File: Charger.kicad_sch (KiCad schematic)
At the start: 86 parts, among them J23 Conn_02x07_Odd_Even, Q6 BSC0702LS, Q7 BSC0702LS, Q8 BSC0702LS, Q9 BSC0702LS, U2 LV2862XDDC, U27 BQ25756RRVR

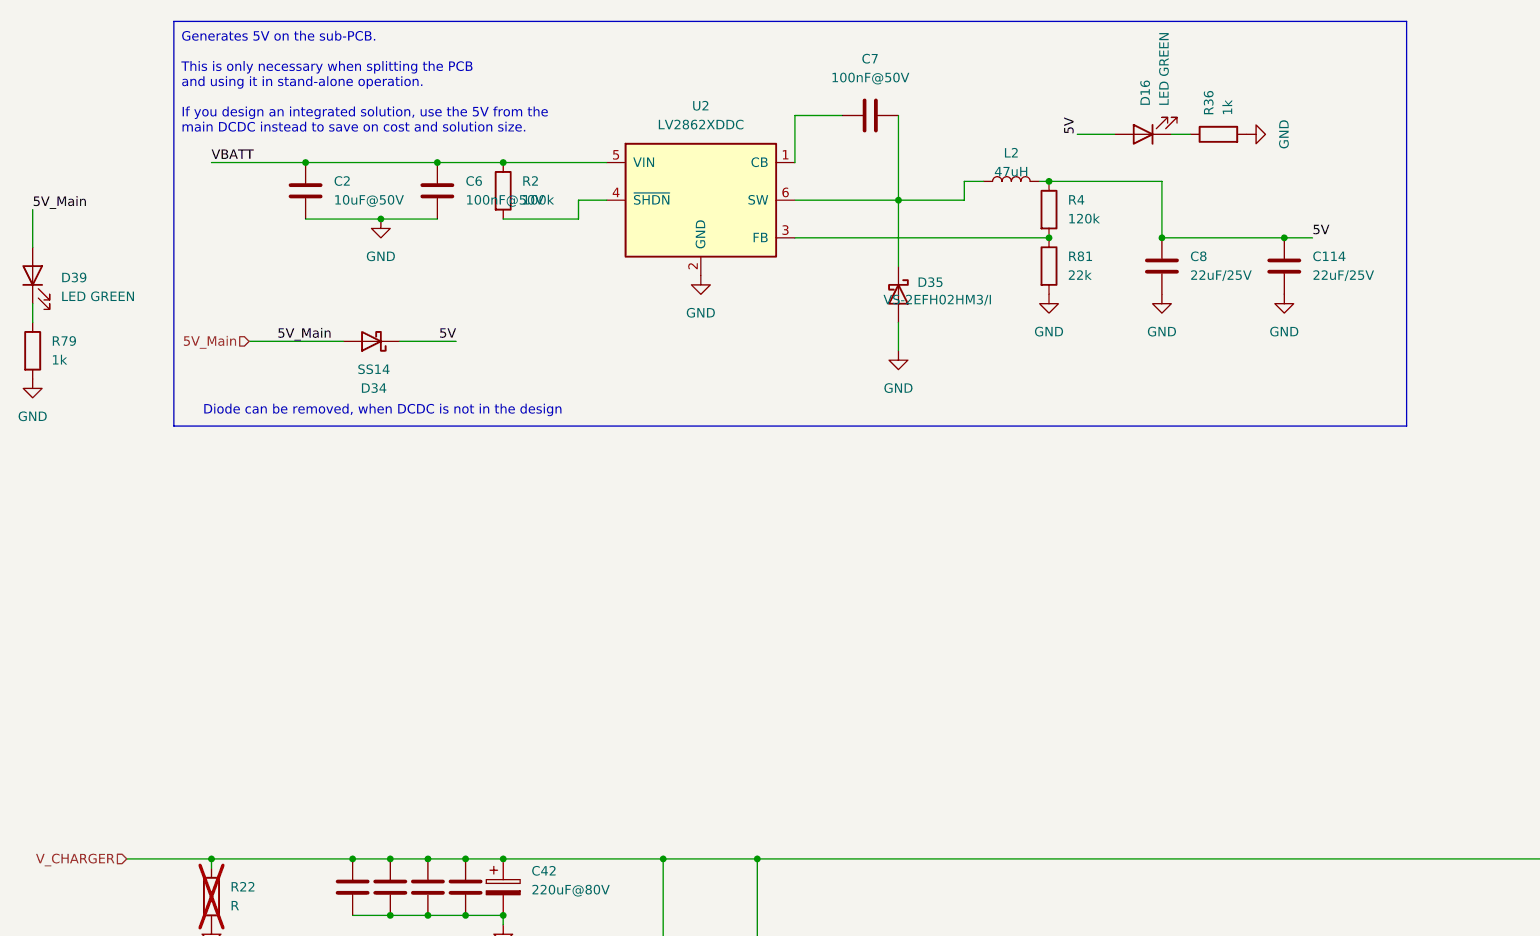
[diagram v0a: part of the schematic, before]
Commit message: wip
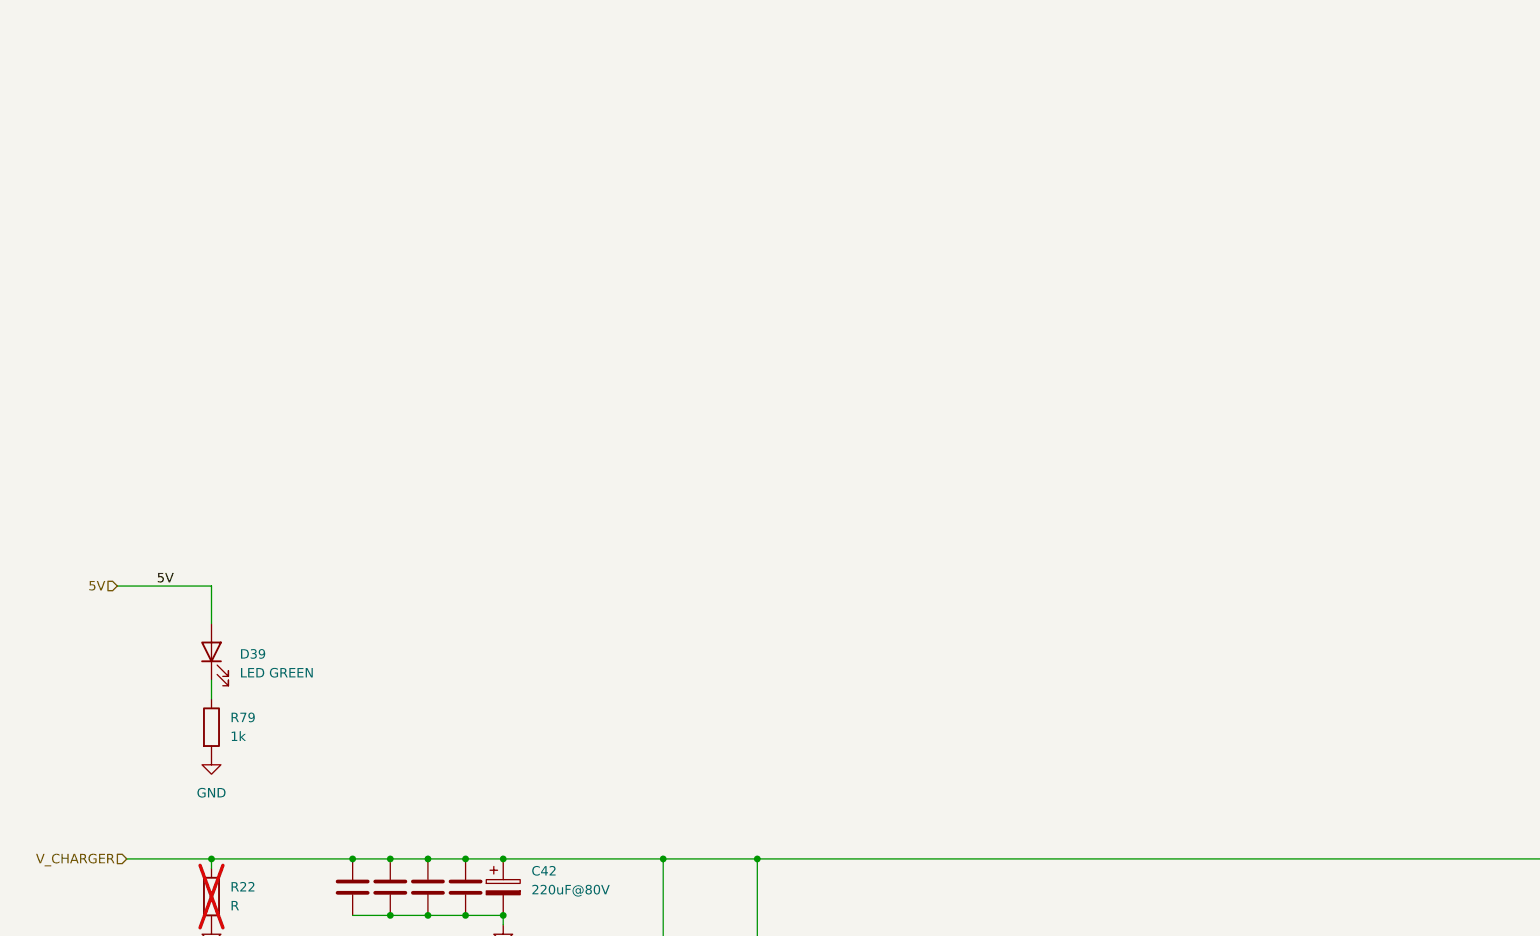
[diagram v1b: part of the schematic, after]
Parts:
- removed C114, C8: 22uF/25V, Capacitor_SMD:C_0805_2012Metric, symbol Device:C
- removed C2: 10uF@50V, Capacitor_SMD:C_1206_3216Metric, symbol Device:C
- removed C6, C7: 100nF@50V, Capacitor_SMD:C_0402_1005Metric, symbol Device:C
- removed D16: LED GREEN, LED_SMD:LED_0805_2012Metric, symbol Device:LED
- removed D34: SS14, Diode_SMD:D_SMA, symbol Diode:SS14
- removed D35: VS-2EFH02HM3/I, Diode_SMD:D_SMF, symbol Device:D_Schottky
- removed L2: 47uH, Inductor_SMD:L_Sunlord_SWPA5040S, symbol Device:L
- removed R2: 100k, Resistor_SMD:R_0402_1005Metric, symbol Device:R
- removed R36: 1k, Resistor_SMD:R_0805_2012Metric, symbol Device:R
- removed R4: 120k, Resistor_SMD:R_0603_1608Metric, symbol Device:R
- removed R81: 22k, Resistor_SMD:R_0603_1608Metric, symbol Device:R
- removed U2: LV2862XDDC, Package_TO_SOT_SMD:SOT-23-6, symbol Regulator_Switching:LV2862XDDC
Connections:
- net 5V_Main is gone; now on net 5V: D39.2 (A)
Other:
- note removed: "Diode can be removed, when DCDC is not in the design"
- note removed: "Generates 5V on the sub-PCB. This is only necessary when splitting the PCB and using it in stand-alone operation. If you design an integrated solution, use the 5V from the main DCDC instead to save on cost and solution size."
- moved on the sheet: D39, R79

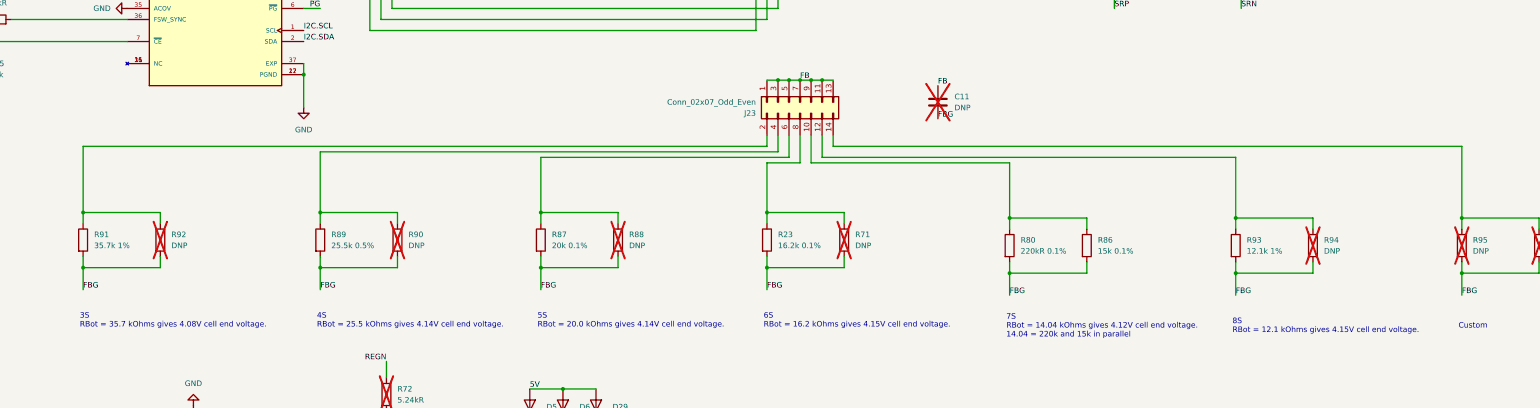
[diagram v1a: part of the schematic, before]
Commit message: wip
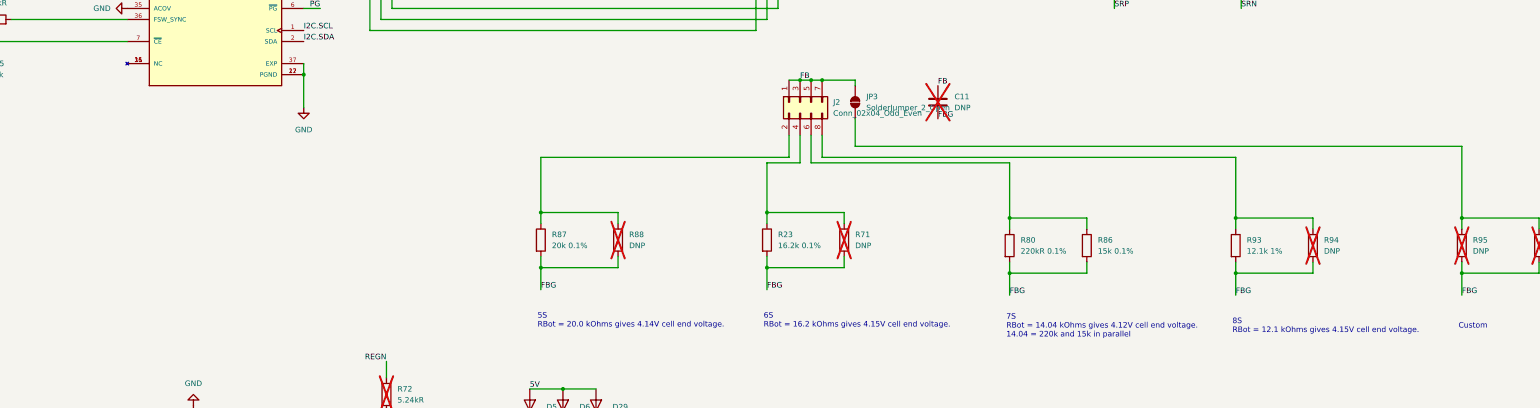
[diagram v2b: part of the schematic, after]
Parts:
- removed J23: Conn_02x07_Odd_Even, Connector_PinHeader_2.54mm:PinHeader_2x07_P2.54mm_Vertical, symbol Connector_Generic:Conn_02x07_Odd_Even
- removed R89: 25.5k 0.5%, Resistor_SMD:R_0603_1608Metric, symbol Device:R
- removed R90, R92: DNP, Resistor_SMD:R_0603_1608Metric, symbol Device:R
- removed R91: 35.7k 1%, Resistor_SMD:R_0603_1608Metric, symbol Device:R
- added J2: Conn_02x04_Odd_Even, Connector_PinHeader_2.54mm:PinHeader_2x04_P2.54mm_Vertical, symbol Connector_Generic:Conn_02x04_Odd_Even
- added JP3: SolderJumper_2_Open, Jumper:SolderJumper-2_P1.3mm_Open_Pad1.0x1.5mm, symbol Jumper:SolderJumper_2_Open
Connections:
- net FB: now also J2.1 (Pin_1), J2.3 (Pin_3), J2.5 (Pin_5), J2.7 (Pin_7), JP3.2 (B)
- net at R80.1, R86.1: now also J2.6 (Pin_6)
- net at R23.1, R71.1: now also J2.4 (Pin_4)
- net at R93.1, R94.1: now also J2.8 (Pin_8)
- net at R95.1, R96.1: now also JP3.1 (A)
- net at R87.1, R88.1: now also J2.2 (Pin_2)
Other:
- note removed: "3S RBot = 35.7 kOhms gives 4.08V cell end voltage."
- note removed: "4S RBot = 25.5 kOhms gives 4.14V cell end voltage."
